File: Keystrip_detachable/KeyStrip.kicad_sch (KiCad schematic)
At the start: 13 parts, among them J1 JST_06, J2 JST_08, J3 JST_06, J4 JST_06

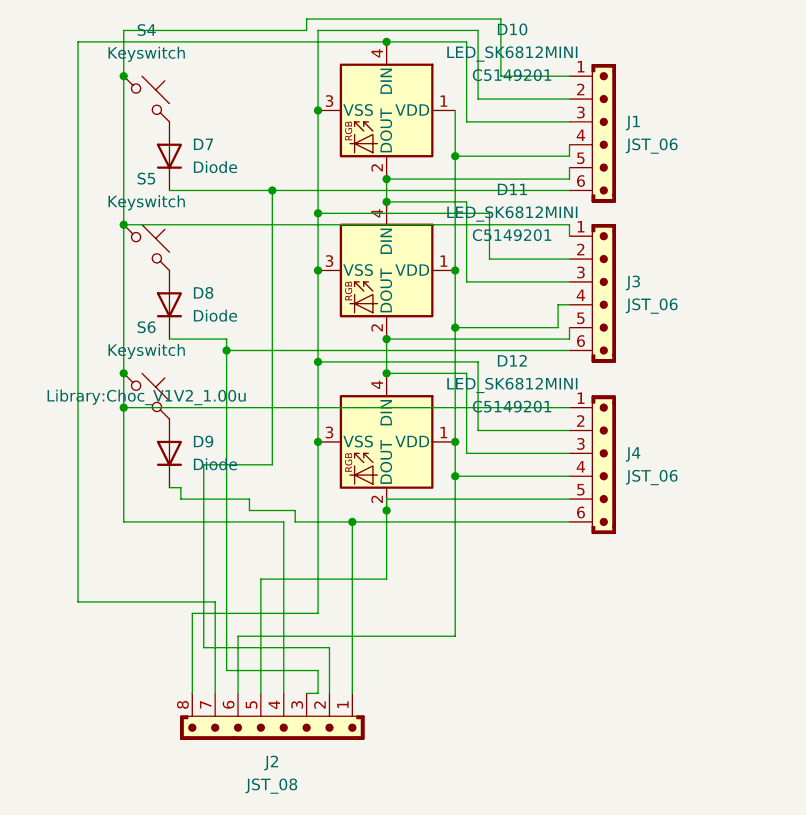
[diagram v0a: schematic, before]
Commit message: ah
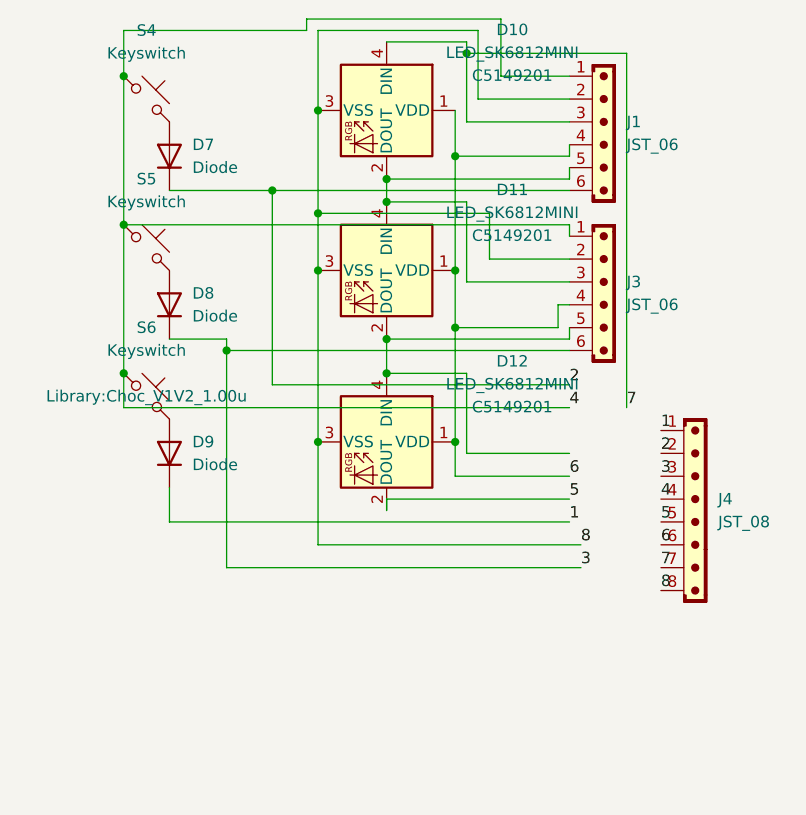
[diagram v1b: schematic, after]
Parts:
- removed J2: JST_08, Library:JST_EH_B8B-EH-A_1x08_P2.50mm_Vertical, symbol PCM_SL_Connectors:JST_08
- removed J4: JST_06, Library:6pin, symbol PCM_SL_Connectors:JST_06
- added J4: JST_08, Library:JST_EH_B8B-EH-A_1x08_P2.50mm_Vertical, symbol PCM_SL_Connectors:JST_08
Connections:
- net 2: now reaches D7.1 (K), J1.6
- net 2: now also J4.2
- net 4: now reaches J1.1, J3.1, S4.1, S5.1, S6.1
- net 4: now also J4.4
- net 1: now reaches D9.1 (K)
- net 1: now also J4.1
- net 3: now reaches D8.1 (K), J3.6
- net 3: now also J4.3
- net 5: now reaches D12.2 (DOUT)
- net 5: now also J4.5
- net 6: now reaches D10.1 (VDD), D11.1 (VDD), D12.1 (VDD), J1.4, J3.4
- net 6: now also J4.6
- net 7: now reaches D10.4 (DIN), J1.3
- net 7: now also J4.7
- net 8: now reaches D10.3 (VSS), D11.3 (VSS), D12.3 (VSS), J1.2, J3.2
- net 8: now also J4.8
